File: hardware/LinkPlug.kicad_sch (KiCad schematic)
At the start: 4 parts, among them J1901 2x05_Horizontal, U1901 THVD24x2

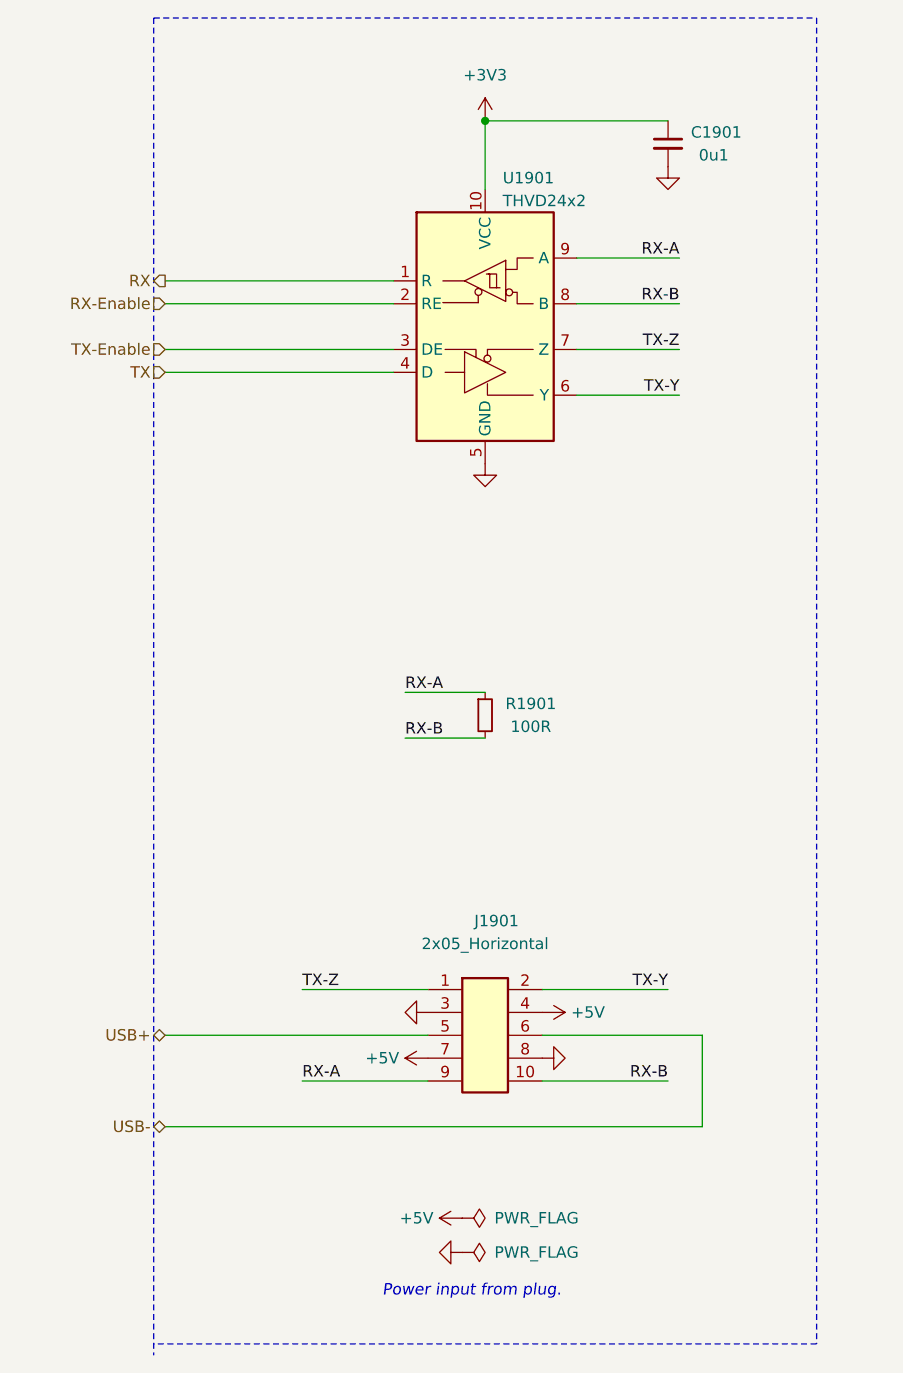
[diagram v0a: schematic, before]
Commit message: Update parts library
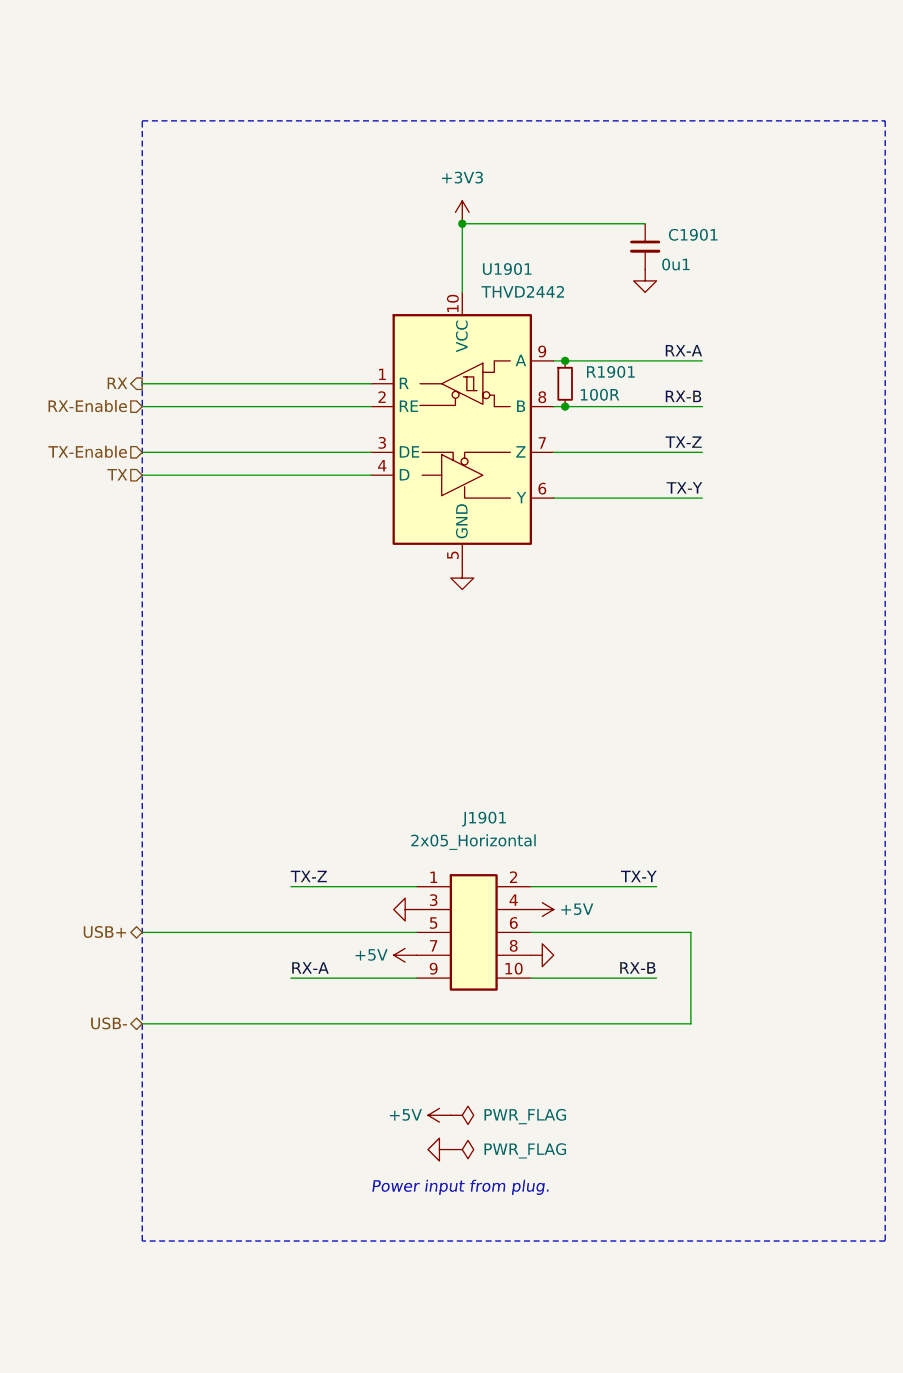
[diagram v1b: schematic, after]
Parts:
- C1901: footprint Capacitor_SMD:C_0603_1608Metric -> V2_Capacitor_SMD:C_0603; symbol Device:C_Small -> V2_Device:C_0603_0u1; Mouser (none) -> 810-CGA3E2X7R1H104MA
- J1901: Mouser (none) -> 649-200211120001T4LF
- R1901: footprint Resistor_SMD:R_0603_1608Metric -> V2_Resistor_SMD:R_0603; symbol Device:R_Small -> V2_Device:R_0603_100R; Mouser (none) -> 71-CRCW0603100RFKEAH
- U1901: value THVD24x2 -> THVD2442; symbol V2_Interface_RS485:THVD24x2 -> V2_Interface_RS485:THVD2442; Mouser (none) -> 595-THVD2442DRCR
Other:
- moved on the sheet: C1901, J1901, R1901, U1901
